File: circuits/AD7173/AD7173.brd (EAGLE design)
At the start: 21.4 x 31.2 mm, 35 parts, among them IC1 AD7173, IC2 ADP1720, IC3 ADP1720ARMZ-5, IC4 ADR445BR, Q1 FA-20H

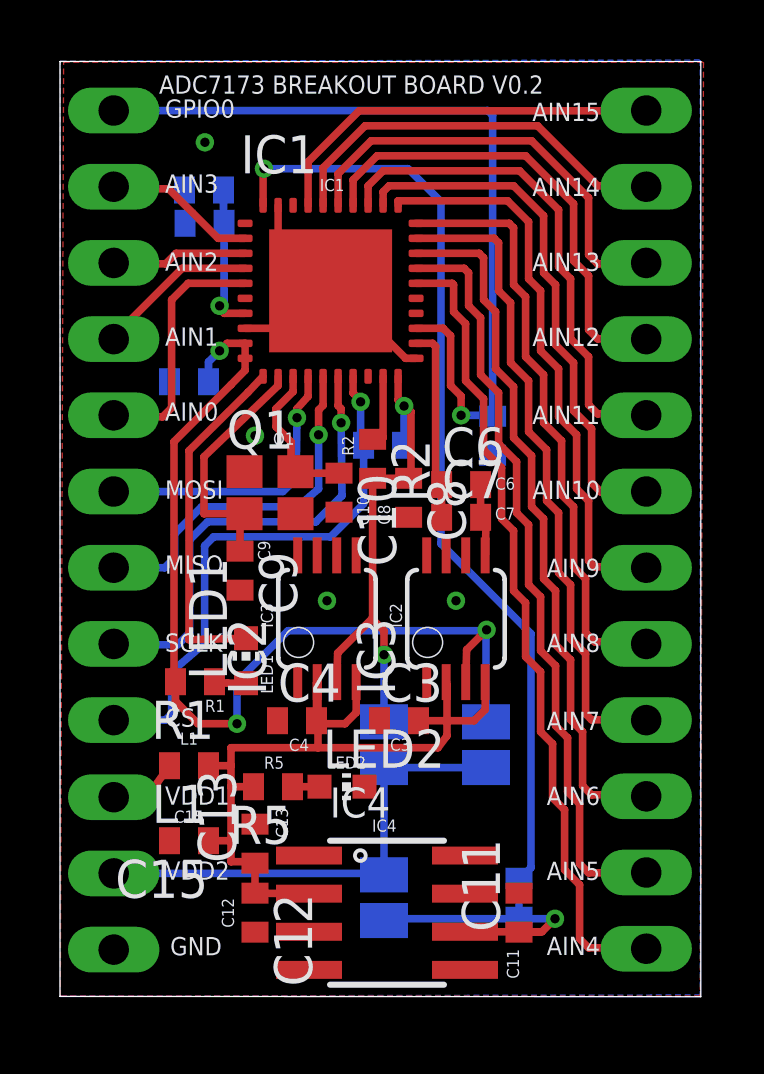
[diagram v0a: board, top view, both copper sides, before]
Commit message: upadted AD7173 breakout board
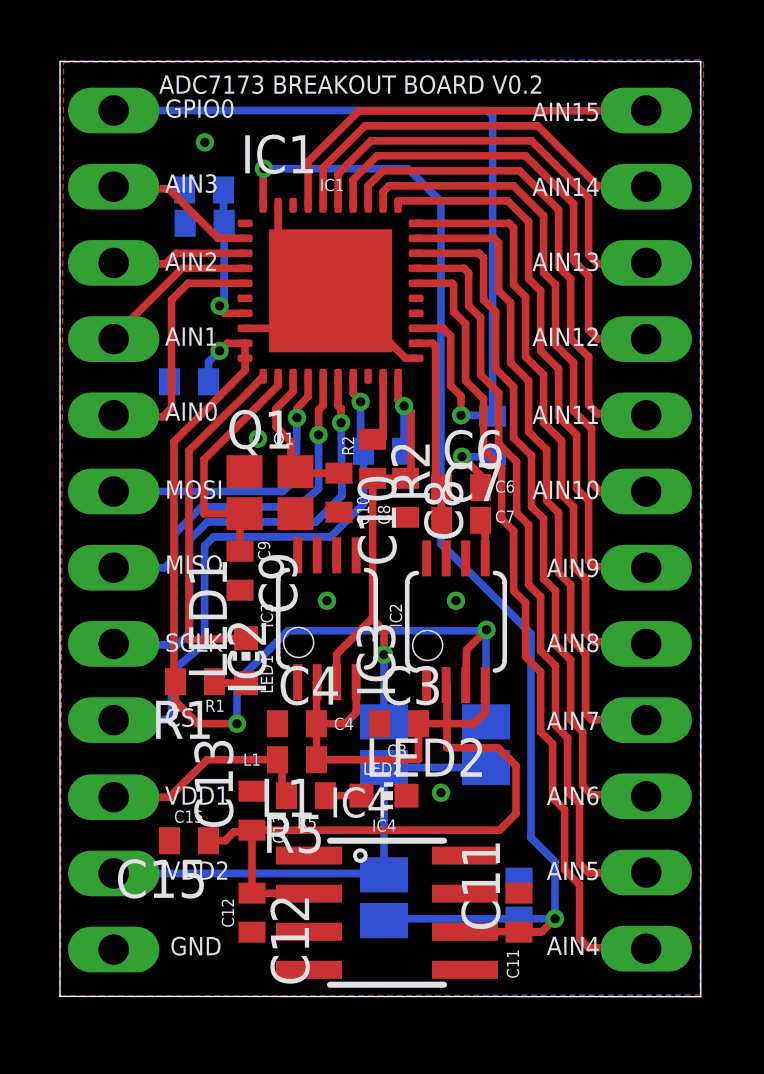
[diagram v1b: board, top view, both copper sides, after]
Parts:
- moved L1 3.61 mm to (7.90, 7.90)
- moved LED2 1.43 mm to (10.8, 6.70)
- moved R5 1.14 mm to (8.20, 6.70)
- moved C13 1.10 mm to (6.40, 6.20)
- moved R4 0.20 mm to (10.8, 18.2)
- moved C6 0.10 mm to (13.4, 17.0)
- moved C12 0.10 mm to (6.40, 2.80)
- moved C3 0.10 mm to (11.3, 9.10)
- moved C4 0.10 mm to (7.90, 9.10)
- moved C7 0.10 mm to (13.4, 15.9)
- moved C8 0.10 mm to (11.5, 16.6)
- moved IC3 0.10 mm to (13.2, 12.5)
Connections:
- net N$30: now also R5.2
- net VIN: no longer R5.2
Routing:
- net VIN: track 28.2 -> 34.1 mm
- net N$30: track 2.40 -> 7.29 mm
- net GND: track 13.5 -> 14.4 mm, vias 4 -> 6

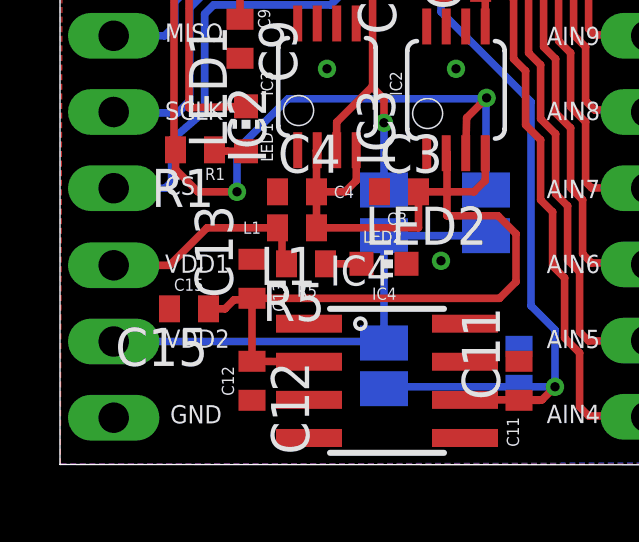
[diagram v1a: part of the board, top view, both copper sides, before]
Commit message: upadted AD7173 breakout board
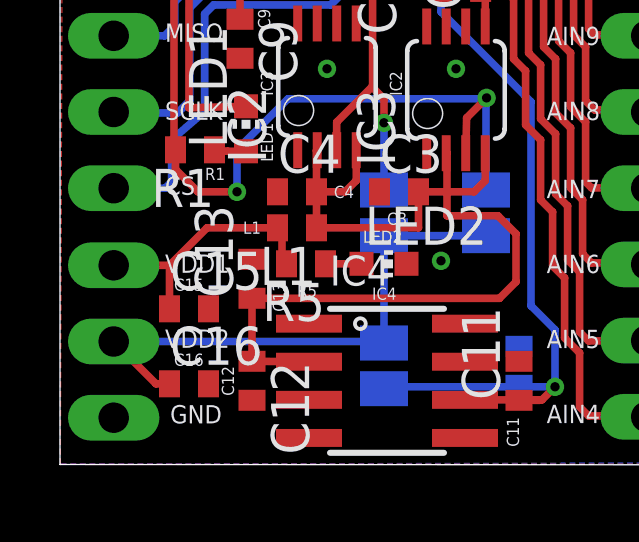
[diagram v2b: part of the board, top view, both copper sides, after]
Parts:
- added C16: 4.7uF, rcl:C0402
- turned C15 to 0 degrees
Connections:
- net GND: now also C16.2
- net N$28: now also C16.1
- net N$30: now also C15.1
- net VIN: no longer C15.1
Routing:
- net N$28: track 16.0 -> 18.4 mm
- net VIN: track 34.1 -> 32.4 mm
- net N$30: track 7.29 -> 8.74 mm
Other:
- board text added: "C16"
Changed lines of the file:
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@@
 <text x="13" y="10.9" size="0.6096" layer="122" font="vector" ratio="10" rot="MR180">AVDD</text>
 <text x="12.4" y="3.9" size="0.4064" layer="122" font="vector" ratio="10" rot="MR270">SJ3</text>
+<text x="3.8" y="3.3" size="0.4064" layer="121" font="vector" ratio="10">C16</text>
 </plain>
 <attributes>
@@
 <element name="C14" library="rcl" package="C0402" value="4.7uF" x="15.3" y="3.3" rot="MR90"/>
 <element name="L1" library="inductors" package="0402" value="BLM15HB121SN1" x="7.9" y="7.9" rot="R180"/>
-<element name="C15" library="rcl" package="C0402" value="0.1uF" x="4.3" y="5.2" rot="R180"/>
+<element name="C15" library="rcl" package="C0402" value="0.1uF" x="4.3" y="5.2"/>
 <element name="SJ1" library="jumper" package="SJ" value="" x="14.2" y="8.4" rot="MR270"/>
 <element name="SJ2" library="jumper" package="SJ" value="" x="10.8" y="8.4" rot="MR270"/>
@@
 <element name="LED2" library="led" package="CHIP-LED0603" value="" x="10.8" y="6.7" rot="R270"/>
 <element name="R5" library="rcl" package="R0402" value="220" x="8.2" y="6.7" rot="R180"/>
+<element name="C16" library="rcl" package="C0402" value="4.7uF" x="4.3" y="2.7"/>
 </elements>
 <signals>
@@
 <wire x1="13.4" y1="18" x2="14.37" y2="18" width="0.254" layer="16"/>
 <wire x1="14.37" y1="18" x2="14.42" y2="18.05" width="0.254" layer="16"/>
+<contactref element="C16" pad="2"/>
 <wire x1="15.3" y1="3.95" x2="15.3" y2="3.45" width="0" layer="19" extent="1-16"/>
 </signal>
@@
 <contactref element="C13" pad="1"/>
 <contactref element="L1" pad="1"/>
-<contactref element="C15" pad="1"/>
 <wire x1="6.4" y1="5.55" x2="6.4" y2="3.45" width="0.254" layer="1"/>
-<wire x1="4.95" y1="5.2" x2="5.5" y2="5.2" width="0.254" layer="1"/>
-<wire x1="5.5" y1="5.2" x2="5.8" y2="5.5" width="0.254" layer="1"/>
-<wire x1="5.8" y1="5.5" x2="6.45" y2="5.5" width="0.254" layer="1"/>
-<wire x1="6.45" y1="5.5" x2="6.4" y2="5.55" width="0.254" layer="1"/>
 <wire x1="6.4" y1="5.55" x2="14.65" y2="5.55" width="0.254" layer="1"/>
 <wire x1="14.65" y1="5.55" x2="15.2" y2="6.1" width="0.254" layer="1"/>
@@
 <wire x1="7.4" y1="7.7" x2="7.4" y2="6.85" width="0.254" layer="1"/>
 <wire x1="7.4" y1="6.85" x2="7.55" y2="6.7" width="0.254" layer="1"/>
+<contactref element="C15" pad="1"/>
+<wire x1="3.65" y1="5.2" x2="3.65" y2="6.65" width="0.254" layer="1"/>
 </signal>
 <signal name="N$28">
@@
 <wire x1="10.8" y1="4.062" x2="10.8" y2="7.638" width="0.254" layer="16"/>
 <wire x1="10.8" y1="7.638" x2="14.2" y2="7.638" width="0.254" layer="16"/>
+<contactref element="C16" pad="1"/>
+<wire x1="3.65" y1="2.7" x2="3.2" y2="2.7" width="0.254" layer="1"/>
+<wire x1="3.2" y1="2.7" x2="1.79" y2="4.11" width="0.254" layer="1"/>
 </signal>
 <signal name="N$31">
